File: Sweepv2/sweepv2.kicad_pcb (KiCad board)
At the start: 2 copper layers, 217.3 x 86.9 mm, 49 parts, among them J1 AudioJack4dpb, J2 AudioJack4dpb, SW10 SW_Push, SW11 SW_Push, SW11_r1 SW_Push, SW12 SW_Push, SW12_r1 SW_Push, SW13_r1 SW_Push, SW14 SW_Push, SW15 SW_Push, SW15_r1 SW_Push, SW16 SW_Push, SW16_r1 SW_Push, SW17 SW_Push, SW17_r1 SW_Push, SW18 SW_Push, SW18_r1 SW_Push, SW2 SW_Push, SW20 SW_Push, SW20_r1 SW_Push, SW21 SW_Push, SW21_r1 SW_Push, SW2_r1 SW_Push, SW3 SW_Push, SW3_r1 SW_Push, SW4 SW_Push, SW4_r1 SW_Push, SW5 SW_Push, SW5_r1 SW_Push, SW6 SW_Push, SW6_r1 SW_Push, SW7_r1 SW_Push, SW8 SW_Push, SW8_r1 SW_Push, SW9 SW_Push, SW9_r1 SW_Push, U1 ProMicro-kbd, U2 ProMicro-kbd

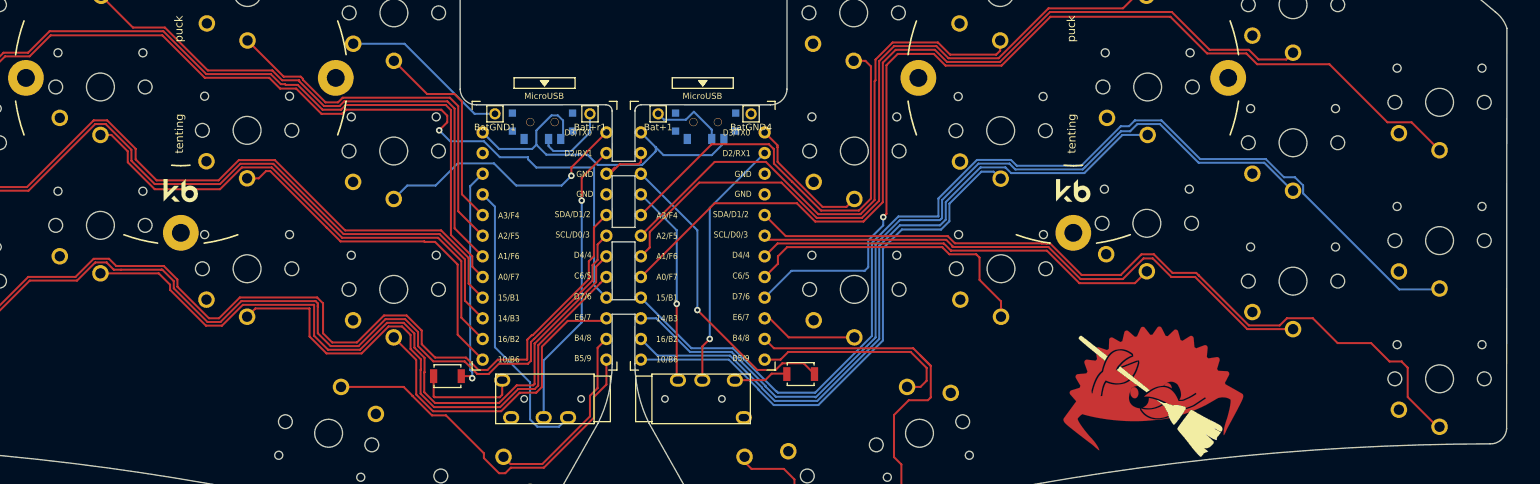
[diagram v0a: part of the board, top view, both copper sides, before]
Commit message: better alignment?
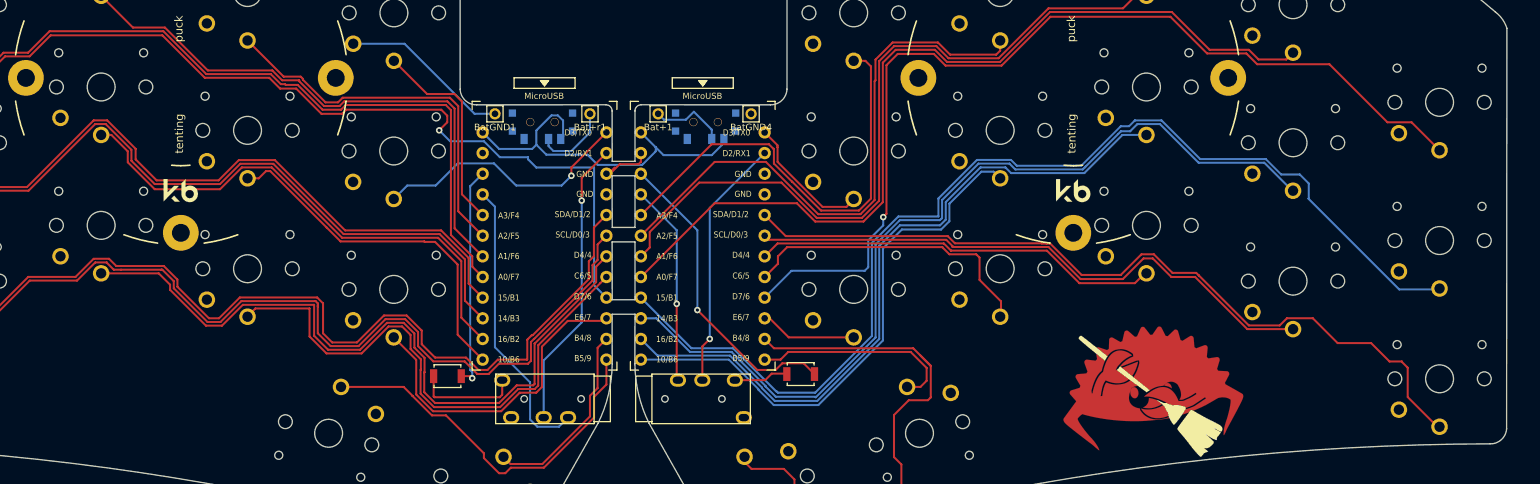
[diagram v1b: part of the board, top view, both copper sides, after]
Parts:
- moved SW15_r1 0.26 mm to (186.5, 56.1)
- moved SW9_r1 0.15 mm to (186.5, 39.1)
- moved SW16_r1 0.10 mm to (168.6, 61.5)
- moved SW10 0.09 mm to (58.0, 39.1)
- moved SW16 0.09 mm to (58.0, 56.1)
- moved SW12_r1 0.08 mm to (150.5, 47.0)
- moved SW17_r1 0.08 mm to (150.5, 64.0)
- moved SW11_r1 0.07 mm to (168.6, 44.5)
- moved SW11 0.05 mm to (76.0, 44.5)
- moved SW17 0.05 mm to (76.0, 61.5)
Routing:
- net Switch6_r: track 134.6 -> 135.2 mm
